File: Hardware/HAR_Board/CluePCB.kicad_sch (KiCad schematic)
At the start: 4 parts

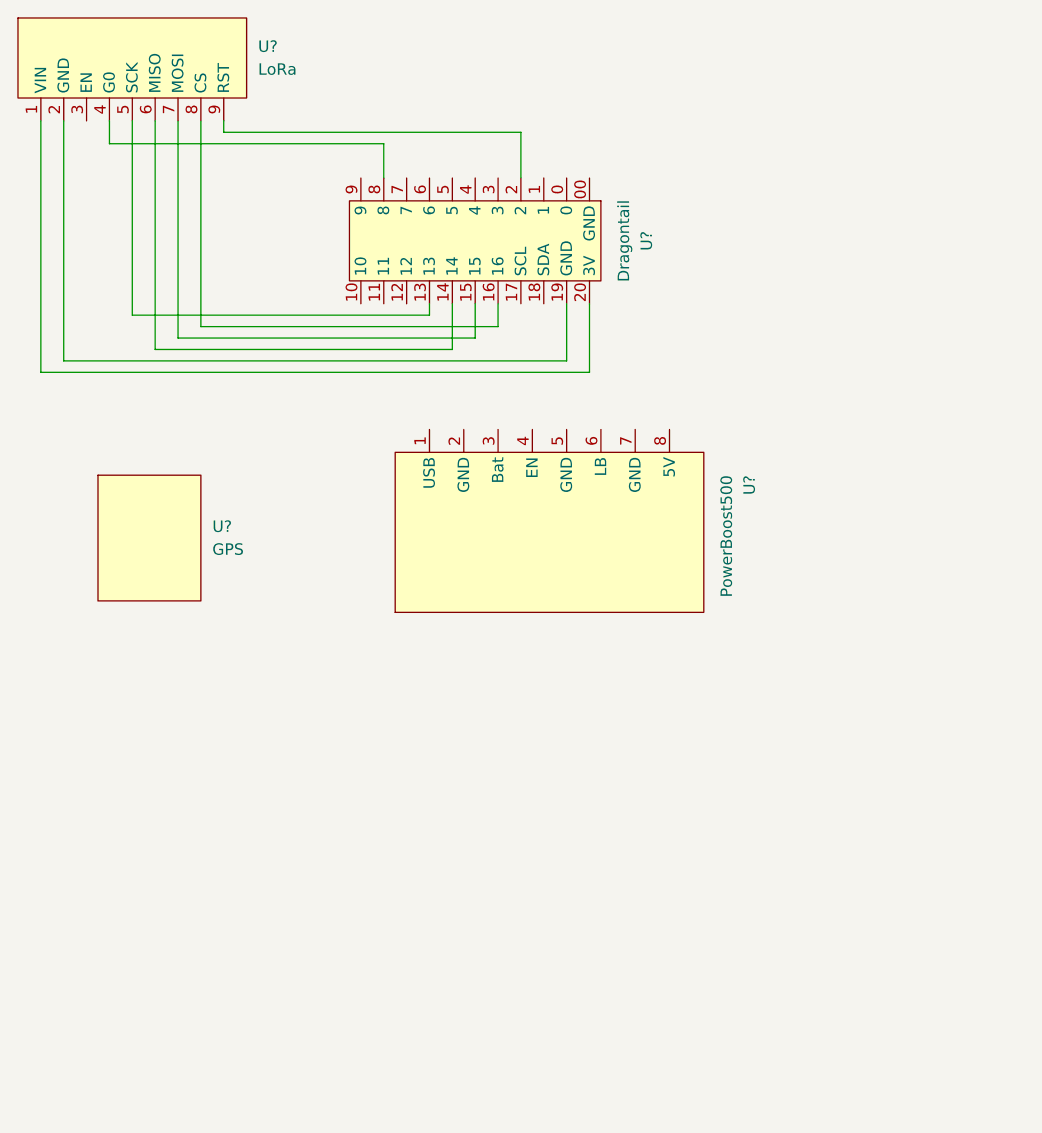
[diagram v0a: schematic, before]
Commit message: Add files via upload
New voltage divider changes
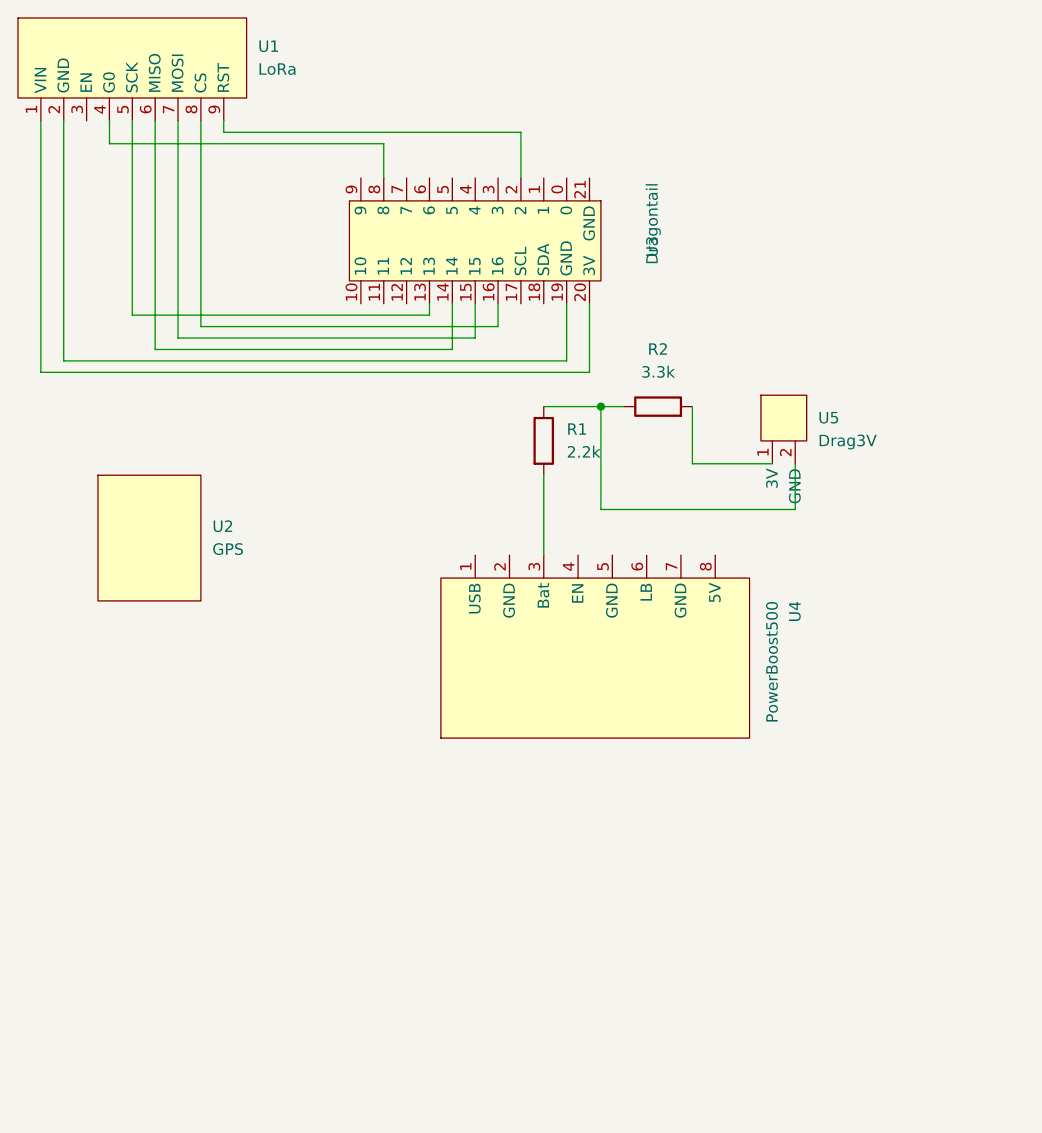
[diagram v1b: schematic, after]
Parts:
- added R1: 2.2k, Resistor_THT:R_Axial_DIN0204_L3.6mm_D1.6mm_P5.08mm_Horizontal, symbol Device:R
- added R2: 3.3k, Resistor_THT:R_Axial_DIN0204_L3.6mm_D1.6mm_P5.08mm_Horizontal, symbol Device:R
- added U5: Drag3V, HABET_Lib:Dragon3V, symbol HABET_Lib:Drag3V
- gave numbers to parts that had none: 4
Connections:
- net at U4.3 (Bat): now also R1.2
- new net: R1.1, R2.1
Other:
- moved on the sheet: U4
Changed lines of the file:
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@@
 (kicad_sch (version 20211123) (generator eeschema)
   (paper "A4")
+  (junction (at 245.11 73.66) (diameter 0) (color 0 0 0 0)
+  )
   (wire (pts (xy 182.88 69.85) (xy 182.88 41.91))
     (stroke (width 0) (type default) (color 0 0 0 0))
@@
     (stroke (width 0) (type default) (color 0 0 0 0))
   )
+  (wire (pts (xy 245.11 85.09) (xy 266.7 85.09))
+    (stroke (width 0) (type default) (color 0 0 0 0))
+  )
+  (wire (pts (xy 266.7 80.01) (xy 266.7 85.09))
+    (stroke (width 0) (type default) (color 0 0 0 0))
+  )
   (wire (pts (xy 231.14 62.23) (xy 231.14 66.04))
     (stroke (width 0) (type default) (color 0 0 0 0))
@@
     (stroke (width 0) (type default) (color 0 0 0 0))
   )
+  (wire (pts (xy 238.76 81.28) (xy 238.76 90.17))
+    (stroke (width 0) (type default) (color 0 0 0 0))
+  )
   (wire (pts (xy 190.5 41.91) (xy 190.5 44.45))
     (stroke (width 0) (type default) (color 0 0 0 0))
@@
     (stroke (width 0) (type default) (color 0 0 0 0))
   )
+  (wire (pts (xy 245.11 73.66) (xy 245.11 85.09))
+    (stroke (width 0) (type default) (color 0 0 0 0))
+  )
   (wire (pts (xy 198.12 41.91) (xy 198.12 66.04))
     (stroke (width 0) (type default) (color 0 0 0 0))
   )
+  (wire (pts (xy 255.27 80.01) (xy 255.27 73.66))
+    (stroke (width 0) (type default) (color 0 0 0 0))
+  )
   (wire (pts (xy 241.3 62.23) (xy 241.3 68.58))
     (stroke (width 0) (type default) (color 0 0 0 0))
   )
+  (wire (pts (xy 238.76 73.66) (xy 245.11 73.66))
+    (stroke (width 0) (type default) (color 0 0 0 0))
+  )
+  (wire (pts (xy 264.16 80.01) (xy 255.27 80.01))
+    (stroke (width 0) (type default) (color 0 0 0 0))
+  )
   (wire (pts (xy 243.84 62.23) (xy 243.84 69.85))
     (stroke (width 0) (type default) (color 0 0 0 0))
@@
     (stroke (width 0) (type default) (color 0 0 0 0))
   )
+  (wire (pts (xy 245.11 73.66) (xy 247.65 73.66))
+    (stroke (width 0) (type default) (color 0 0 0 0))
+  )
   (wire (pts (xy 231.14 66.04) (xy 198.12 66.04))
     (stroke (width 0) (type default) (color 0 0 0 0))
@@
     (stroke (width 0) (type default) (color 0 0 0 0))
   )
+  (symbol (lib_id "Device:R") (at 251.46 73.66 90) (unit 1)
+    (in_bom yes) (on_board yes) (fields_autoplaced)
+    (property "Reference" "R2" (id 0) (at 251.46 67.31 90))
+    (property "Value" "3.3k" (id 1) (at 251.46 69.85 90))
+    (property "Footprint" "Resistor_THT:R_Axial_DIN0204_L3.6mm_D1.6mm_P5.08mm_Horizontal" (id 2) (at 251.46 75.438 90)
+      (effects (font (size 1.27 1.27)) hide)
+    )
+    (property "Datasheet" "~" (id 3) (at 251.46 73.66 0)
+      (effects (font (size 1.27 1.27)) hide)
+    )
+    (pin "1")
+    (pin "2")
+  )
+  (symbol (lib_id "HABET_Lib:Drag3V") (at 265.43 71.12 0) (unit 1)
+    (in_bom yes) (on_board yes) (fields_autoplaced)
+    (property "Reference" "U5" (id 0) (at 269.24 74.9299 0)
+      (effects (font (size 1.27 1.27)) (justify left))
+    )
+    (property "Value" "Drag3V" (id 1) (at 269.24 77.4699 0)
+      (effects (font (size 1.27 1.27)) (justify left))
+    )
+    (property "Footprint" "HABET_Lib:Dragon3V" (id 2) (at 265.43 68.58 0)
+      (effects (font (size 1.27 1.27)) hide)
+    )
+    (property "Datasheet" "" (id 3) (at 265.43 66.04 0)
+      (effects (font (size 1.27 1.27)) hide)
+    )
+    (pin "1")
+    (pin "2")
+  )
   (symbol (lib_id "HABET_Lib:GPS") (at 191.77 80.01 0) (unit 1)
     (in_bom yes) (on_board yes) (fields_autoplaced)
-    (property "Reference" "U?" (id 0) (at 201.93 86.9949 0)
+    (property "Reference" "U2" (id 0) (at 201.93 86.9949 0)
       (effects (font (size 1.27 1.27)) (justify left))
     )
@@
   (symbol (lib_id "HABET_Lib:Dragontail") (at 250.19 55.88 270) (unit 1)
     (in_bom yes) (on_board yes) (fields_autoplaced)
-    (property "Reference" "U?" (id 0) (at 250.19 55.245 0))
-    (property "Value" "Dragontail" (id 1) (at 247.65 55.245 0))
-    (property "Footprint" "HABET_Lib:Dragontail" (id 2) (at 251.46 55.88 0)
-      (effects (font (size 1.27 1.27)) hide)
-    )
-    (property "Datasheet" "" (id 3) (at 248.92 54.61 0)
+    (property "Reference" "U3" (id 0) (at 250.825 55.88 0))
+    (property "Value" "Dragontail" (id 1) (at 250.825 53.34 0))
+    (property "Footprint" "HABET_Lib:Dragontail" (id 2) (at 250.19 57.15 0)
+      (effects (font (size 1.27 1.27)) hide)
+    )
+    (property "Datasheet" "" (id 3) (at 251.46 54.61 0)
       (effects (font (size 1.27 1.27)) hide)
     )
     (pin "0")
-    (pin "00")
     (pin "1")
     (pin "10")
@@
     (pin "2")
     (pin "20")
+    (pin "21")
     (pin "3")
     (pin "4")
@@
   (symbol (lib_id "HABET_Lib:LoRa") (at 187.96 24.13 0) (unit 1)
     (in_bom yes) (on_board yes) (fields_autoplaced)
-    (property "Reference" "U?" (id 0) (at 207.01 33.6549 0)
+    (property "Reference" "U1" (id 0) (at 207.01 33.6549 0)
       (effects (font (size 1.27 1.27)) (justify left))
     )
@@
     (pin "9")
   )
-  (symbol (lib_id "HABET_Lib:PowerBoost500") (at 261.62 90.17 270) (unit 1)
+  (symbol (lib_id "HABET_Lib:PowerBoost500") (at 266.7 104.14 270) (unit 1)
     (in_bom yes) (on_board yes)
-    (property "Reference" "U?" (id 0) (at 261.62 81.28 0)
-      (effects (font (size 1.27 1.27)) (justify left))
-    )
-    (property "Value" "PowerBoost500" (id 1) (at 259.08 81.28 0)
-      (effects (font (size 1.27 1.27)) (justify left))
-    )
-    (property "Footprint" "HABET_Lib:Powerboost500" (id 2) (at 265.43 86.36 0)
-      (effects (font (size 1.27 1.27)) hide)
-    )
-    (property "Datasheet" "" (id 3) (at 261.62 77.47 0)
+    (property "Reference" "U4" (id 0) (at 266.7 95.25 0)
+      (effects (font (size 1.27 1.27)) (justify left))
+    )
+    (property "Value" "PowerBoost500" (id 1) (at 264.16 95.25 0)
+      (effects (font (size 1.27 1.27)) (justify left))
+    )
+    (property "Footprint" "HABET_Lib:Powerboost500" (id 2) (at 270.51 100.33 0)
+      (effects (font (size 1.27 1.27)) hide)
+    )
+    (property "Datasheet" "" (id 3) (at 266.7 91.44 0)
       (effects (font (size 1.27 1.27)) hide)
     )
@@
     (pin "8")
   )
+  (symbol (lib_id "Device:R") (at 238.76 77.47 0) (unit 1)
+    (in_bom yes) (on_board yes) (fields_autoplaced)
+    (property "Reference" "R1" (id 0) (at 241.3 76.1999 0)
+      (effects (font (size 1.27 1.27)) (justify left))
+    )
+    (property "Value" "2.2k" (id 1) (at 241.3 78.7399 0)
+      (effects (font (size 1.27 1.27)) (justify left))
+    )
+    (property "Footprint" "Resistor_THT:R_Axial_DIN0204_L3.6mm_D1.6mm_P5.08mm_Horizontal" (id 2) (at 236.982 77.47 90)
+      (effects (font (size 1.27 1.27)) hide)
+    )
+    (property "Datasheet" "~" (id 3) (at 238.76 77.47 0)
+      (effects (font (size 1.27 1.27)) hide)
+    )
+    (pin "1")
+    (pin "2")
+  )
   (sheet_instances
     (path "/" (page "1"))
   )
   (symbol_instances
+    (path "/f2e02e40-b0f6-4d99-a71d-3ac4f1b845ca"
+      (reference "R1") (unit 1) (value "2.2k") (footprint "Resistor_THT:R_Axial_DIN0204_L3.6mm_D1.6mm_P5.08mm_Horizontal")
+    )
+    (path "/0228f8a9-46dc-46b3-a0c2-4b38290ad621"
+      (reference "R2") (unit 1) (value "3.3k") (footprint "Resistor_THT:R_Axial_DIN0204_L3.6mm_D1.6mm_P5.08mm_Horizontal")
+    )
+    (path "/e89ba419-1f6c-4927-ae55-2707f89537ba"
+      (reference "U1") (unit 1) (value "LoRa") (footprint "HABET_Lib:LoRa")
+    )
     (path "/c7dabde8-8bab-432f-a281-bb0485a78429"
-      (reference "U?") (unit 1) (value "GPS") (footprint "HABET_Lib:GPS")
+      (reference "U2") (unit 1) (value "GPS") (footprint "HABET_Lib:GPS")
     )
     (path "/d7a5a19b-fe6e-43f6-818d-21d8dd99a019"
-      (reference "U?") (unit 1) (value "Dragontail") (footprint "HABET_Lib:Dragontail")
-    )
-    (path "/e89ba419-1f6c-4927-ae55-2707f89537ba"
-      (reference "U?") (unit 1) (value "LoRa") (footprint "HABET_Lib:LoRa")
+      (reference "U3") (unit 1) (value "Dragontail") (footprint "HABET_Lib:Dragontail")
     )
     (path "/ec4681fd-ad45-4d21-9f18-09355a2e5b88"
-      (reference "U?") (unit 1) (value "PowerBoost500") (footprint "HABET_Lib:Powerboost500")
-    )
-  )
+      (reference "U4") (unit 1) (value "PowerBoost500") (footprint "HABET_Lib:Powerboost500")
+    )
+    (path "/1d973257-91f4-48d4-9e9e-51d77eb1499a"
+      (reference "U5") (unit 1) (value "Drag3V") (footprint "HABET_Lib:Dragon3V")
+    )
+  )
